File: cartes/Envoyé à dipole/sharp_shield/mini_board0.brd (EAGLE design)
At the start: 44.9 x 37.5 mm, 22 parts, among them U1 MCP2551

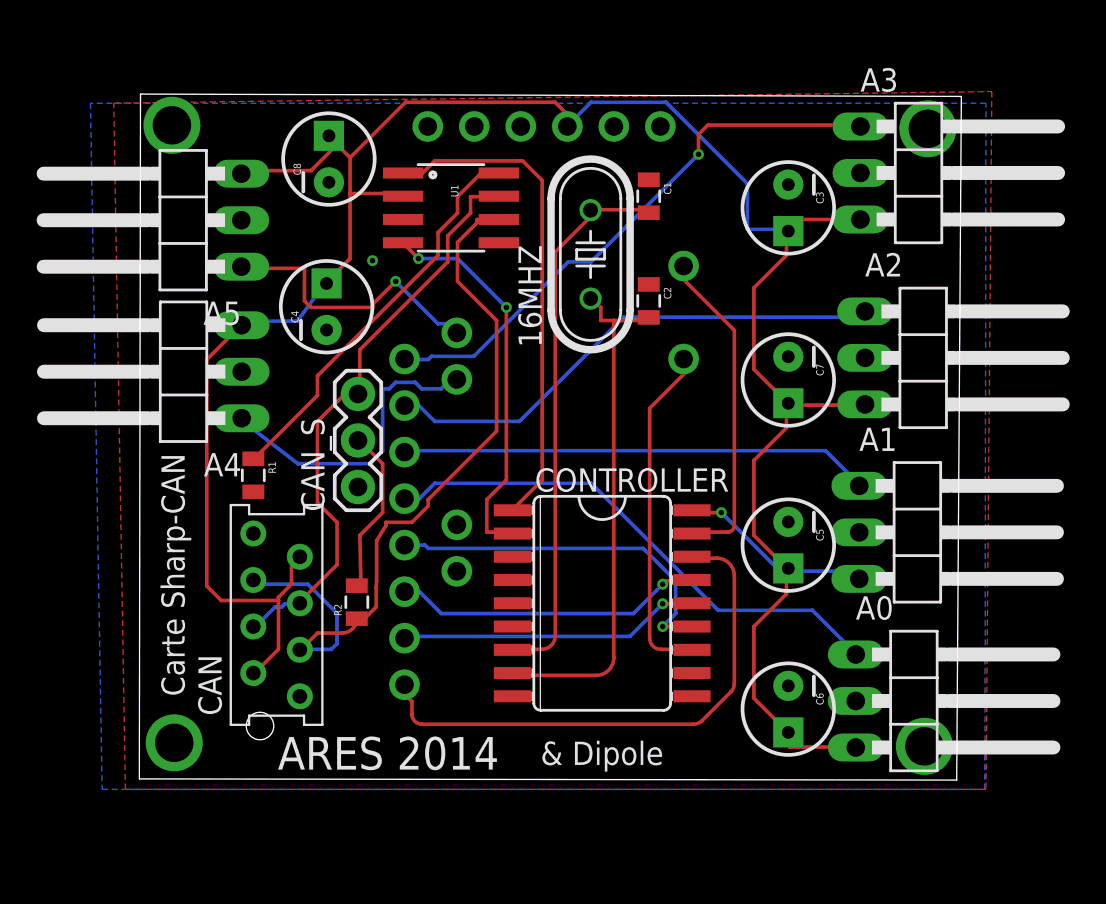
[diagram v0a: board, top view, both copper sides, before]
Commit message: ajout  cartes à envoyer
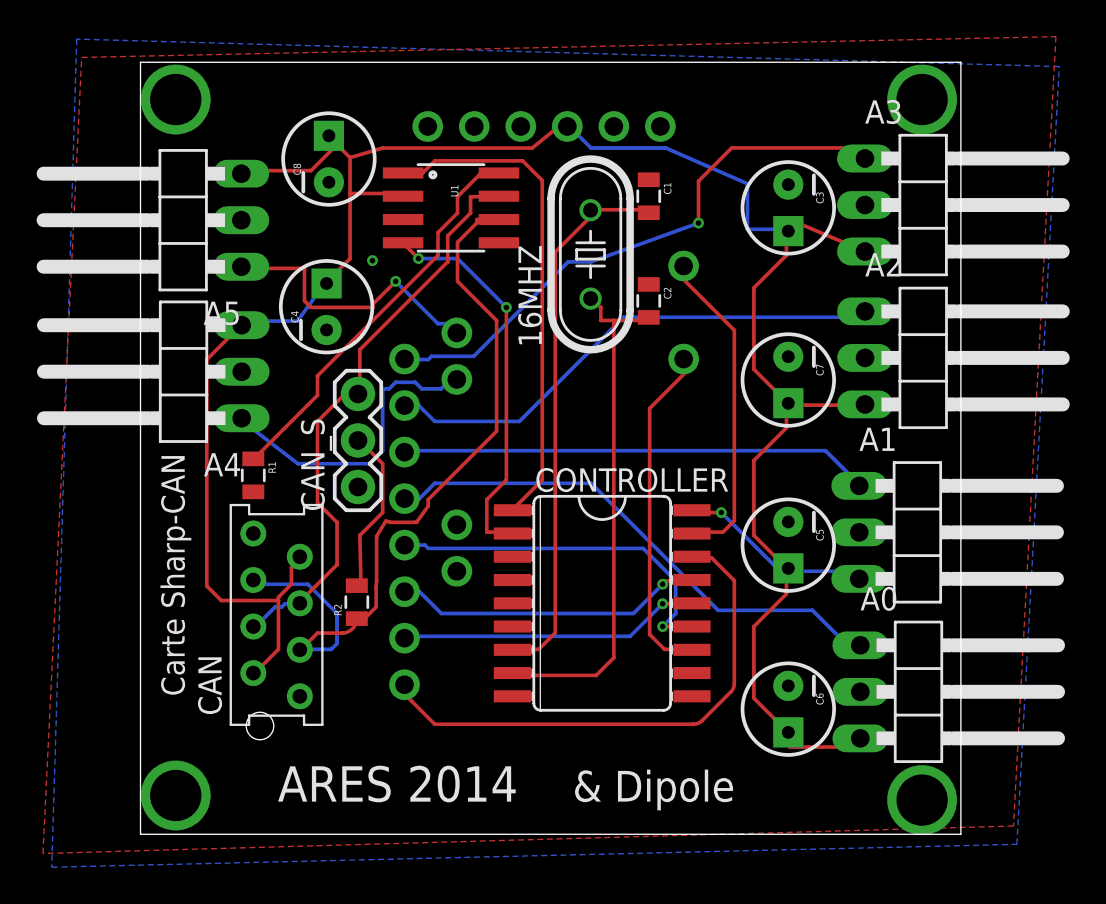
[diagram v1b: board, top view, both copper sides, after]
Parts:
- moved A3 1.77 mm to (44.2, 45.2)
- moved A0 0.56 mm to (43.9, 18.7)
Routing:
- net VCC: track 138.4 -> 136.7 mm
- net CAN_CS: track 29.4 -> 28.9 mm
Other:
- board size 44.9 x 37.5 mm -> 44.8 x 42.2 mm
